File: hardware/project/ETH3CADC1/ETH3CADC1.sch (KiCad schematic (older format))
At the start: 2 parts

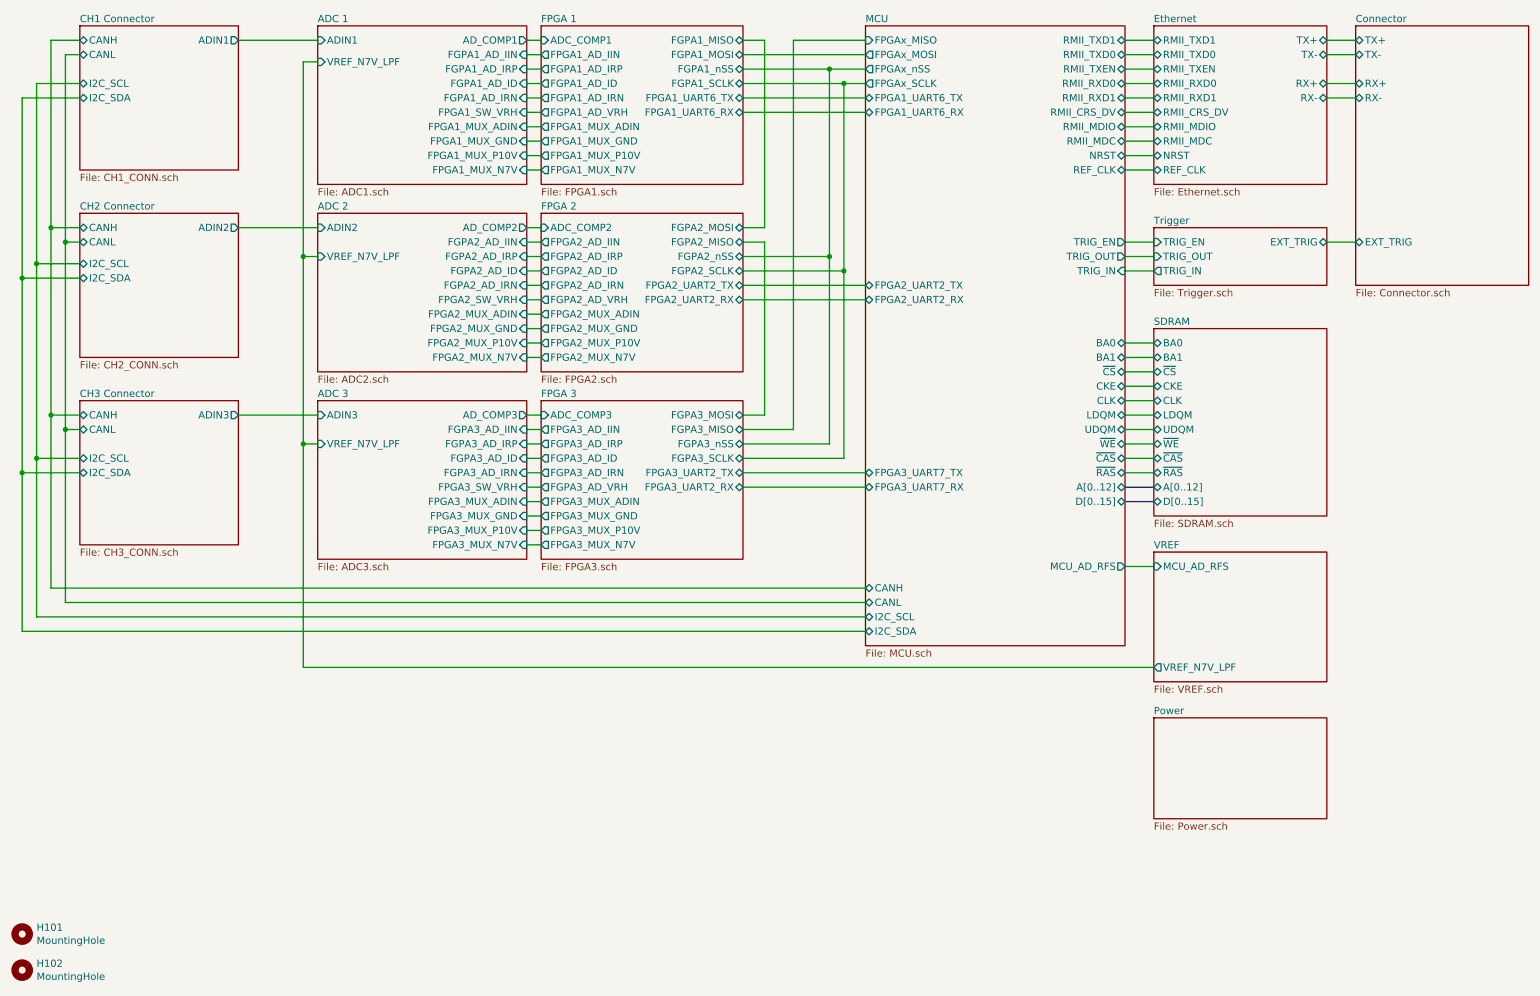
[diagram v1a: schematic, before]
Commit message: Software development.
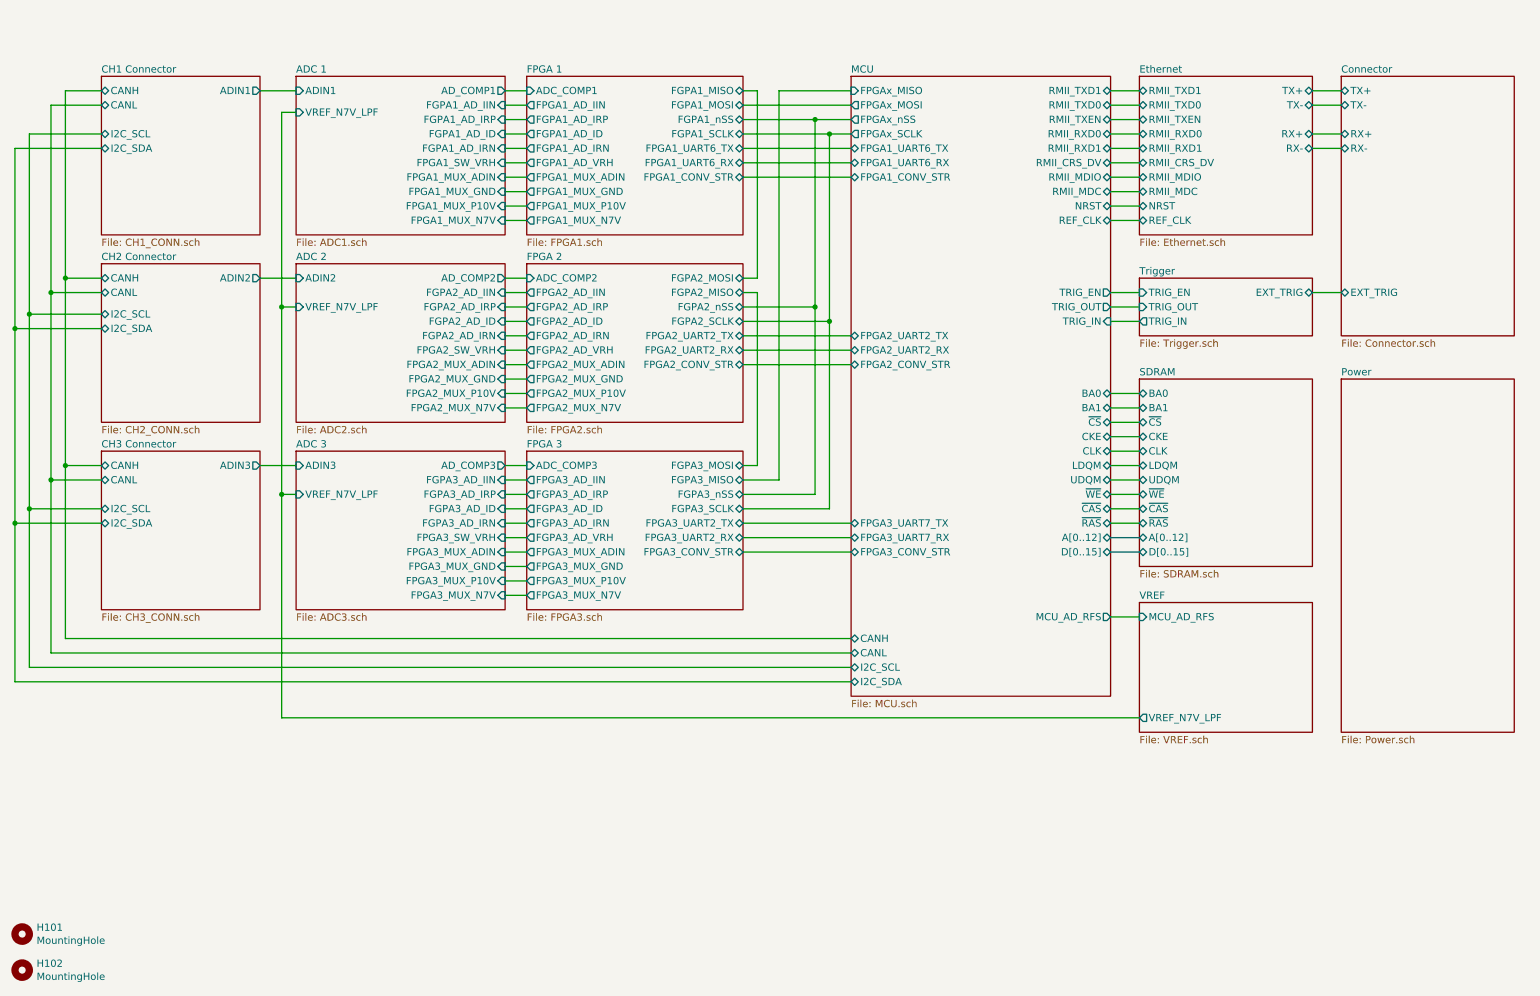
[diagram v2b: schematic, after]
